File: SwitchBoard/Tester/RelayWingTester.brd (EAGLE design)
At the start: 70.8 x 63.5 mm, 18 parts

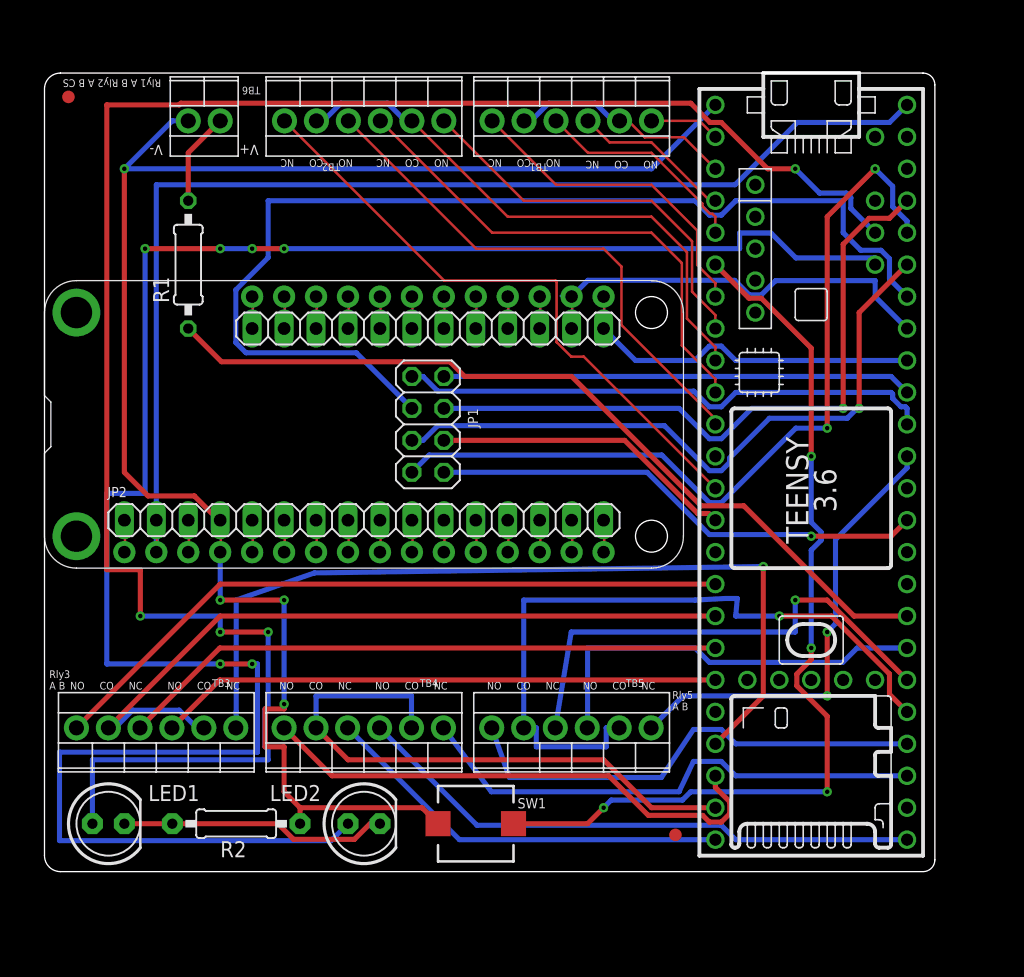
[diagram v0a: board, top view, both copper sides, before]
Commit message: Adding Rev B changes for the Tester
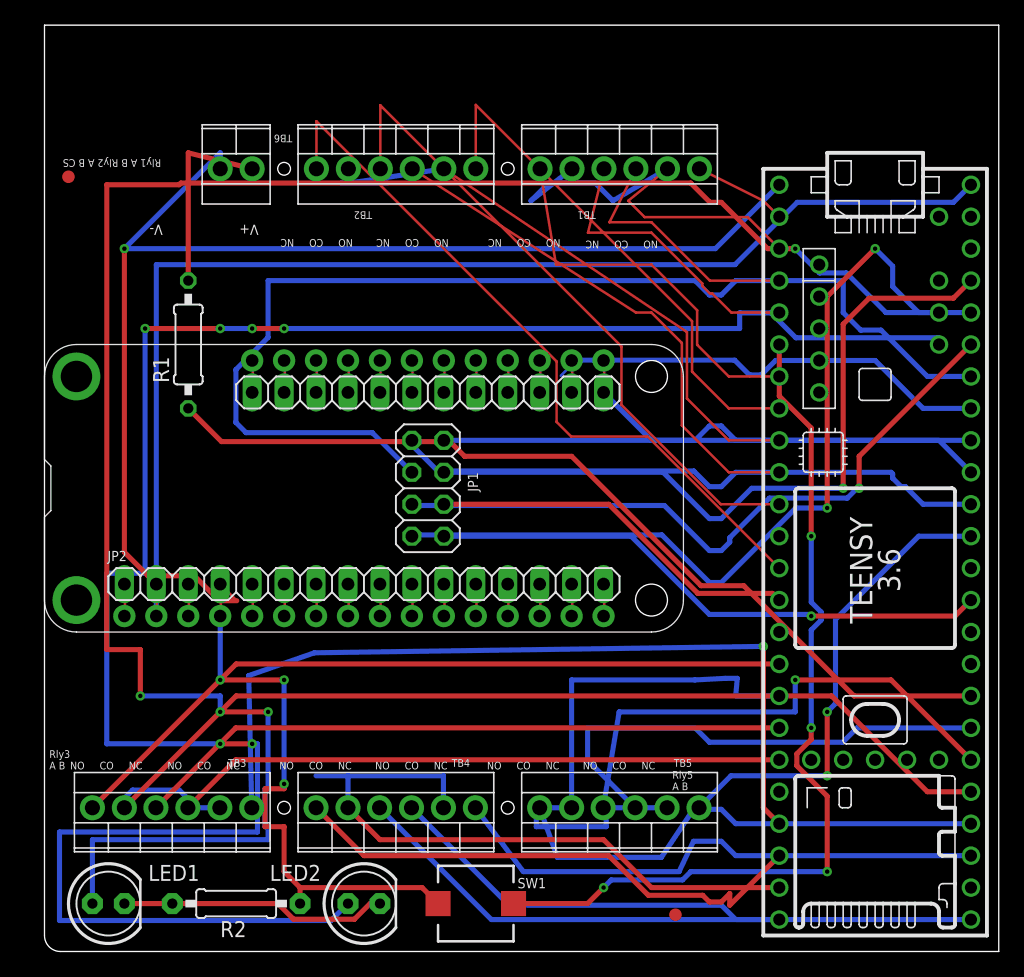
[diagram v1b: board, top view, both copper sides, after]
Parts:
- moved U$4 8.13 mm to (66.0, 33.0)
- moved TB5 7.41 mm to (45.7, 11.4)
- moved TB4 6.84 mm to (27.9, 11.4)
- moved TB3 6.48 mm to (10.2, 11.4)
- moved R1 6.35 mm to (11.4, 48.3)
- moved U$3 6.35 mm to (50.2, 2.92)
- moved LED1 6.35 mm to (5.08, 3.81)
- moved LED2 6.35 mm to (25.4, 3.81)
- moved R2 6.35 mm to (15.2, 3.81)
- moved SW1 6.35 mm to (34.3, 3.81)
- moved U$2 6.35 mm to (1.91, 61.6)
- moved TB1 5.39 mm to (45.7, 62.2)
- moved MS1 5.08 mm to (0.00, 25.4)
- moved JP1 5.08 mm to (30.5, 36.8)
- moved JP2 5.08 mm to (25.4, 29.2)
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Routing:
- net N$17: track 18.0 -> 34.4 mm
- net GND: track 134.4 -> 147.9 mm
- net N$31: track 42.2 -> 52.6 mm
- net N$28: track 31.4 -> 41.6 mm
- net N$33: track 49.2 -> 58.1 mm
- net N$54: track 7.40 -> 15.4 mm
- net N$24: track 12.8 -> 20.2 mm
- net N$49: track 32.7 -> 39.3 mm
- net N$25: track 17.2 -> 23.2 mm
- net N$47: track 56.9 -> 62.8 mm
- net N$60: track 53.3 -> 58.9 mm
- net N$62: track 24.2 -> 29.8 mm
- net N$63: track 39.5 -> 45.1 mm
- net N$56: track 37.4 -> 43.0 mm
- net N$2: track 28.7 -> 34.3 mm
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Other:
- board size 70.8 x 63.5 mm -> 75.9 x 73.7 mm
